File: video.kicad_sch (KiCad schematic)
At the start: 12 parts, among them J1 Conn_Coaxial, J2 Conn_Coaxial, Q1 2N4401, U6 TMS9918A, Y1 10.738635MHz

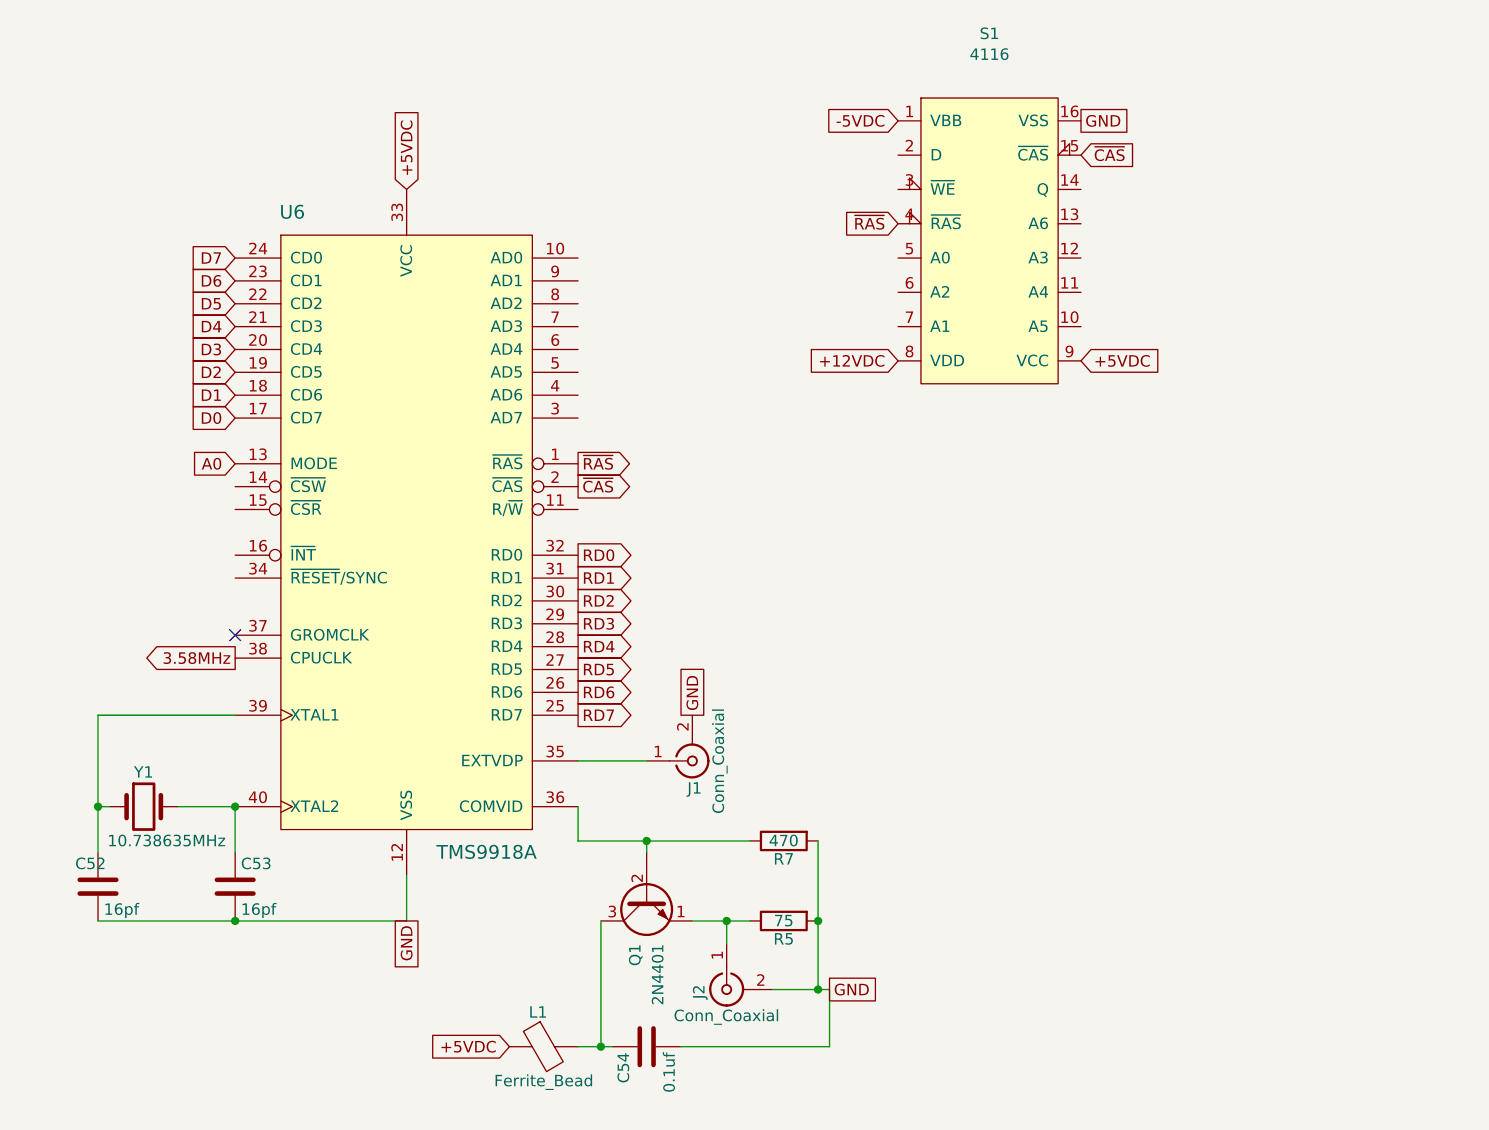
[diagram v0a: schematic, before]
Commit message: Add files via upload
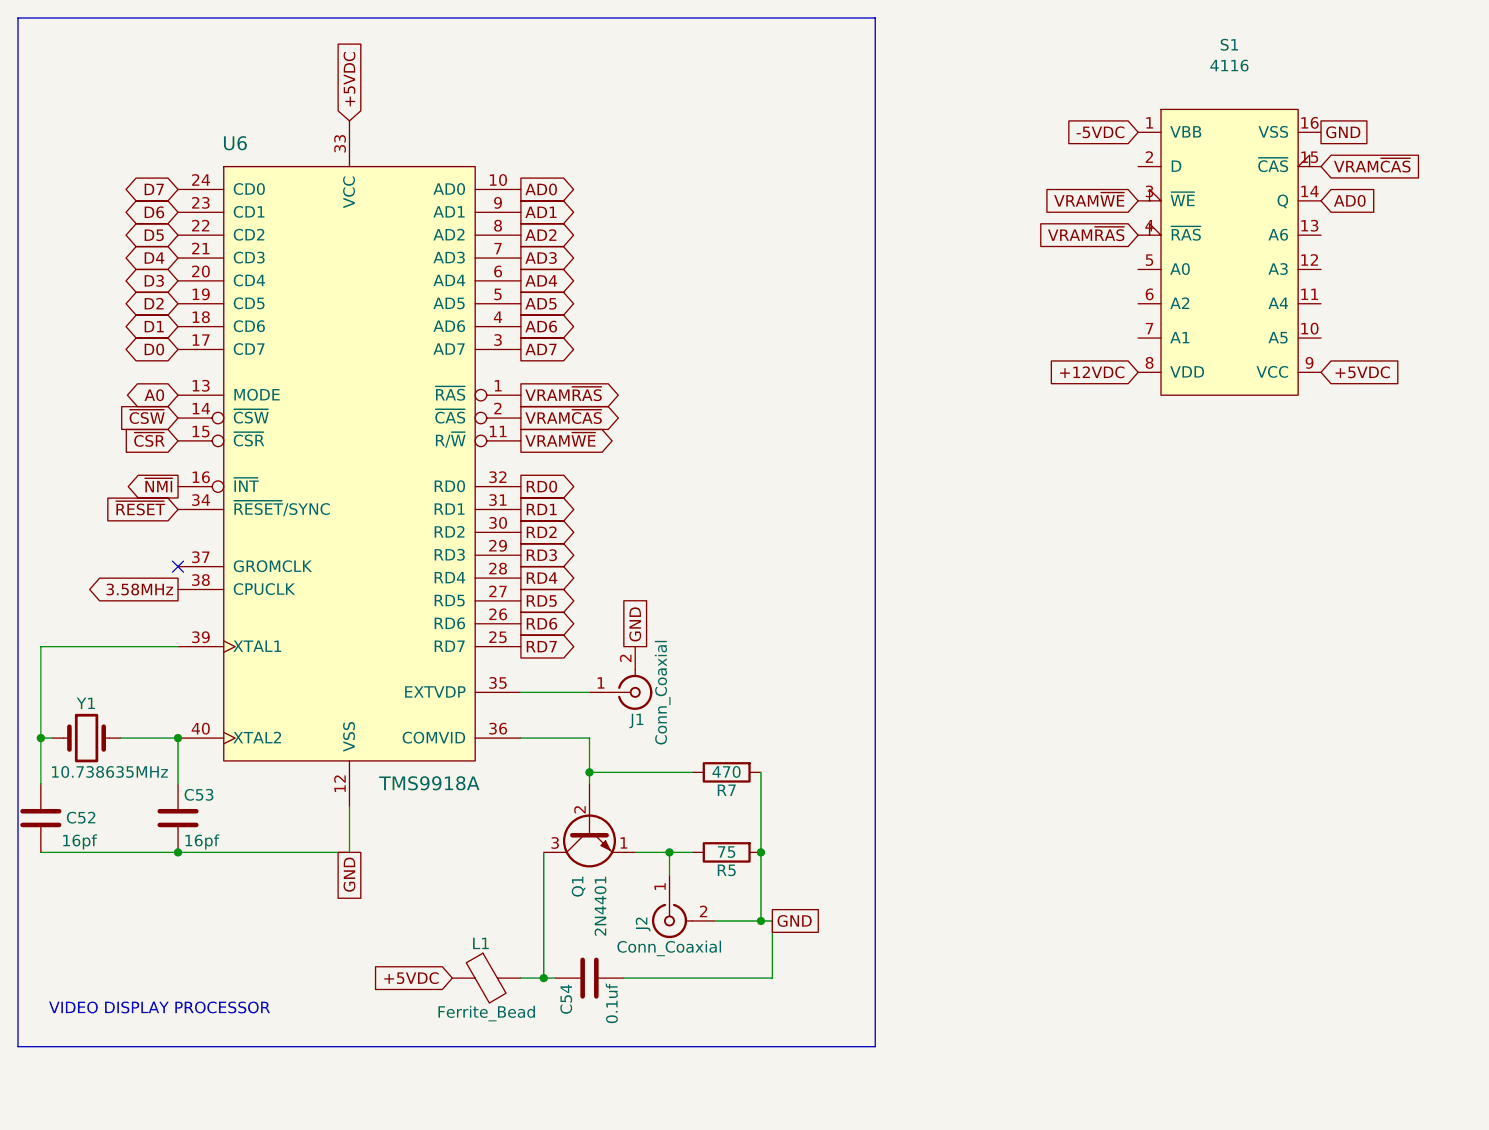
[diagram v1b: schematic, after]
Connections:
- net AD0: now reaches U6.10 (AD0)
- net AD0: now also S1.14 (Q)
- net VRAM~{WE}: now reaches U6.11 (R/~{W})
- net VRAM~{WE}: now also S1.3 (~{WE})
- net ~{CSW}: now reaches U6.14 (~{CSW})
- net ~{CSR}: now reaches U6.15 (~{CSR})
- net ~{NMI}: now reaches U6.16 (~{INT})
- net AD7: now reaches U6.3 (AD7)
- net ~{RESET}: now reaches U6.34 (~{RESET}/SYNC)
- net AD6: now reaches U6.4 (AD6)
- net AD5: now reaches U6.5 (AD5)
- net AD4: now reaches U6.6 (AD4)
- net AD3: now reaches U6.7 (AD3)
- net AD2: now reaches U6.8 (AD2)
- net AD1: now reaches U6.9 (AD1)
- net ~{CAS} renamed VRAM~{CAS}
- net ~{RAS} renamed VRAM~{RAS}
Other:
- note added: "VIDEO DISPLAY PROCESSOR"
- moved on the sheet: C52, C53, C54, J1, J2, L1, Q1, R5, R7, S1, U6, Y1
